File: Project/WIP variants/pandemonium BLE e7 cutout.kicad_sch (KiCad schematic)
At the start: 134 parts, among them J1 HRO_TYPE-C-31-M-14, J1 TC2030_SWD, J3 78171-0002, J4 Conn_01x02_Female, Q1 2N7002, SW1 RotaryEncoder_Switch, SW2 RotaryEncoder_Switch, SW3 RST, SW4 SW_SPDT, U1 nRF52840_E73-2G4M08S1C, U2 SRV05-4, U6 MAX17048, U7 BQ24075, Y1 32.768 KHz

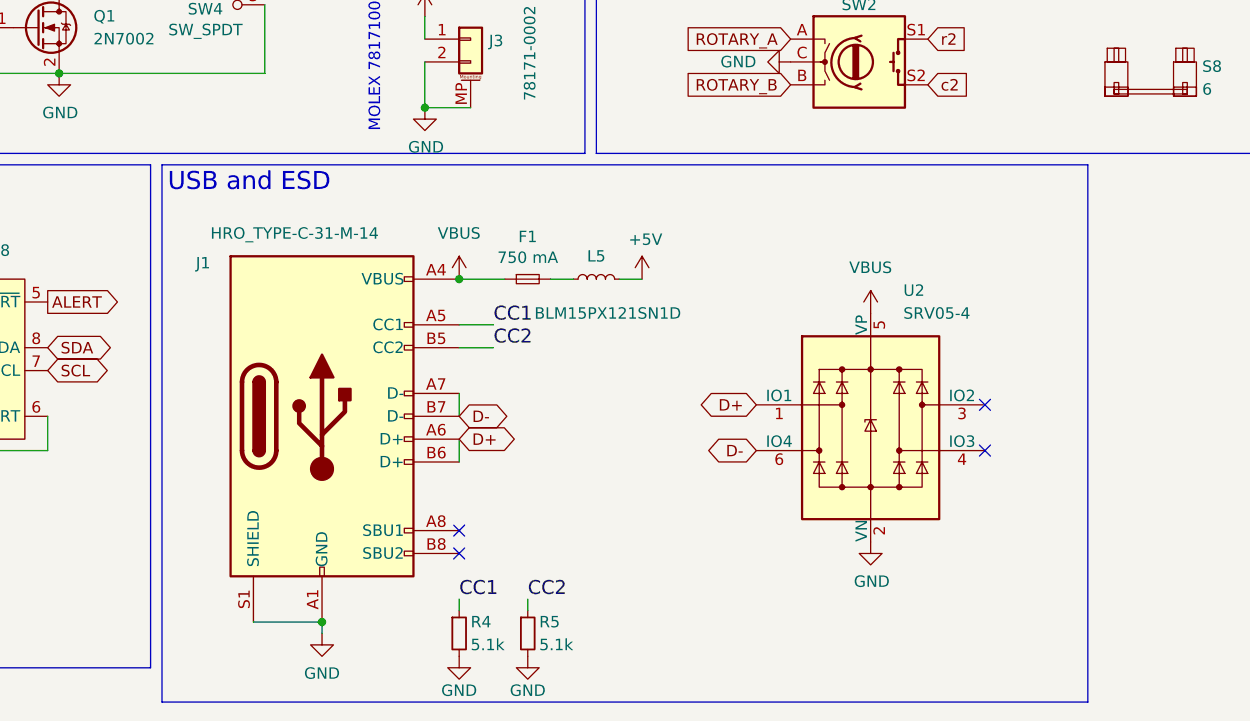
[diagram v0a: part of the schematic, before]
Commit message: BLE & EC edited
requires production files!!
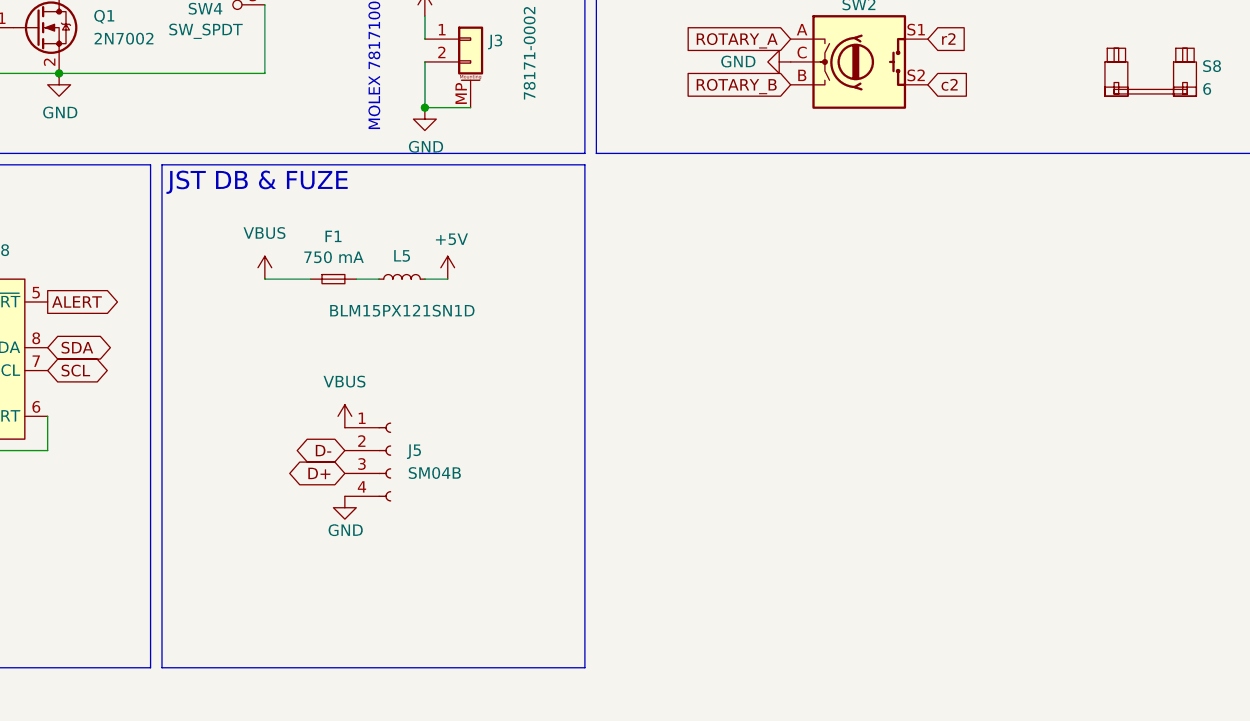
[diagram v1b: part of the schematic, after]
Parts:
- removed J1: HRO_TYPE-C-31-M-14, PCM_marbastlib-various:USB_C_Receptacle_HRO_TYPE-C-31-M-12, symbol Connector:USB_C_Receptacle_USB2.0
- removed R4, R5: 5.1k, Resistor_SMD:R_0402_1005Metric, symbol Device:R_Small
- removed U2: SRV05-4, PCM_marbastlib-various:SOT-23-6-routable, symbol PCM_marbastlib-various:SRV05-4
- added J5: SM04B, Connector_JST:JST_SH_SM04B-SRSS-TB_1x04-1MP_P1.00mm_Horizontal, symbol Connector:Conn_01x04_Female
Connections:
- net D+: now also J5.3 (Pin_3)
- net D-: now also J5.2 (Pin_2)
- net GND: now also J5.4 (Pin_4)
- net VBUS: now also J5.1 (Pin_1)
- no-connect marks 15 -> 11
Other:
- note added: "JST DB & FUZE"
- note removed: "USB and ESD"
- moved on the sheet: F1, L5
